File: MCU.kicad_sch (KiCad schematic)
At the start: 81 parts, among them J13 2068320402, J3 FTSH-107-01-L-D-K, J4 USB_C_Receptacle_USB2.0_16P, Q1 PMOS, Q10 NMOS, SW2 SW_Push, U1 MCP2562-E-SN, U13 TPD2EUSB30, U14 MAX40200AUK, U15 MAX40200AUK, U16 CP2102N-Axx-xQFN20, U4 STM32F103C8Tx, U5 AZ1117-3.3, U6 AZ1117-5.0, Y3 8MHz, Y4 32.768K

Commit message: test
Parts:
- J13: symbol Misc:2068320402 -> Symbols:2068320402
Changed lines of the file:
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@@
 	)
 	(symbol
-		(lib_id "Misc:2068320402")
+		(lib_id "Symbols:2068320402")
 		(at 231.14 124.46 0)
 		(mirror y)

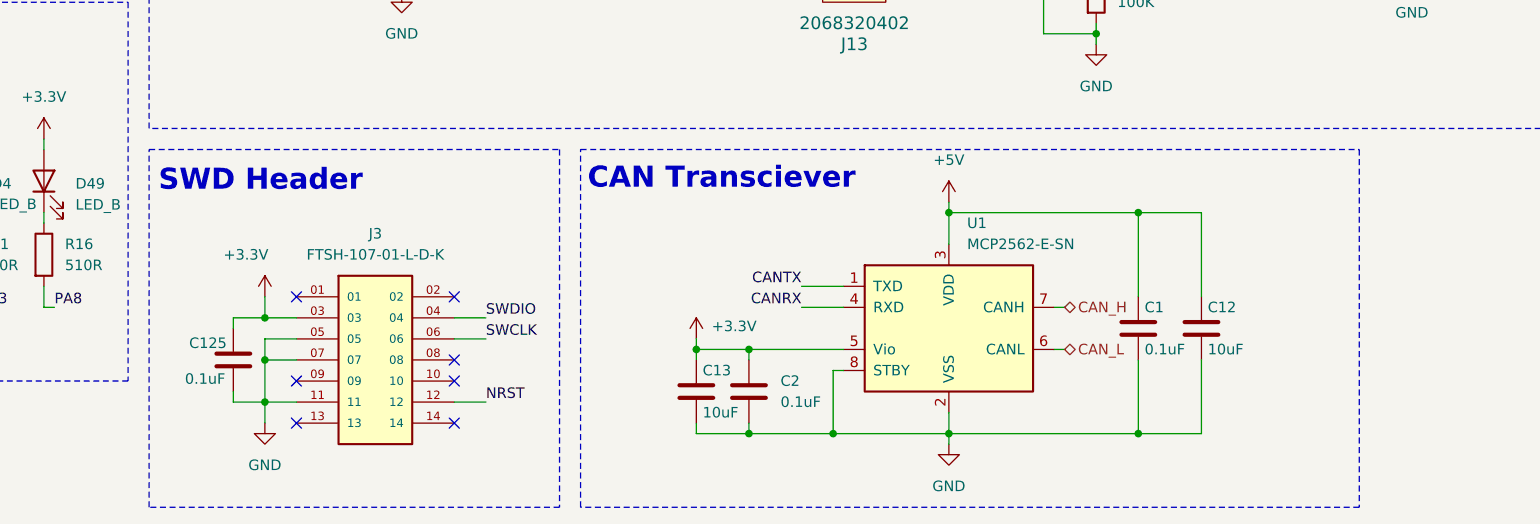
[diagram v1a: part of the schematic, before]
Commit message: library updates
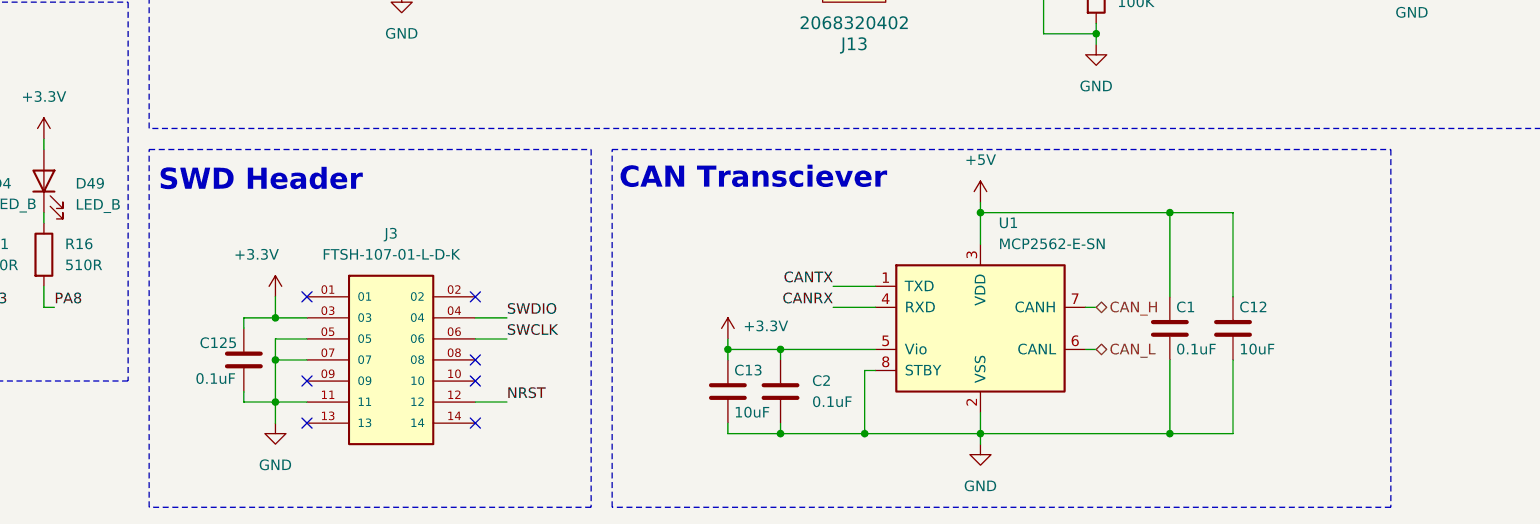
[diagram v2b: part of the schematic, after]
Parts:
- J13: symbol Symbols:2068320402 -> Misc:2068320402
- J3: footprint Connector_Samtec:SAMTEC_FTSH-107-01-L-D-K -> Footprints:SAMTEC_FTSH-107-01-L-D-K; symbol Connector:FTSH-107-01-L-D-K -> Symbols:FTSH-107-01-L-D-K
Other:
- moved on the sheet: C1, C12, C125, C13, C2, J3, U1
